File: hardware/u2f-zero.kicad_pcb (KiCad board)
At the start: 2 copper layers, 40.5 x 14.5 mm, 16 parts, among them SW1 SW_PUSH

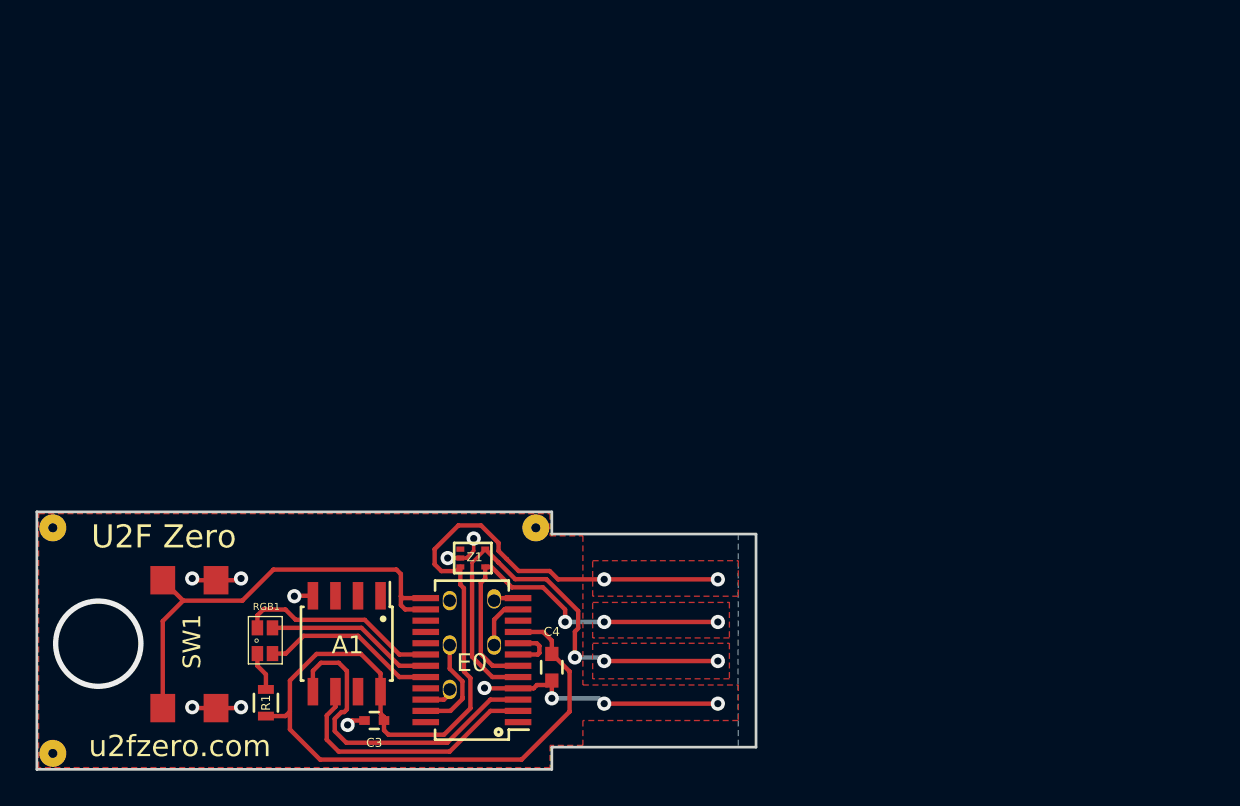
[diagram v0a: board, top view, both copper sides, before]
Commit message: Ensmallen
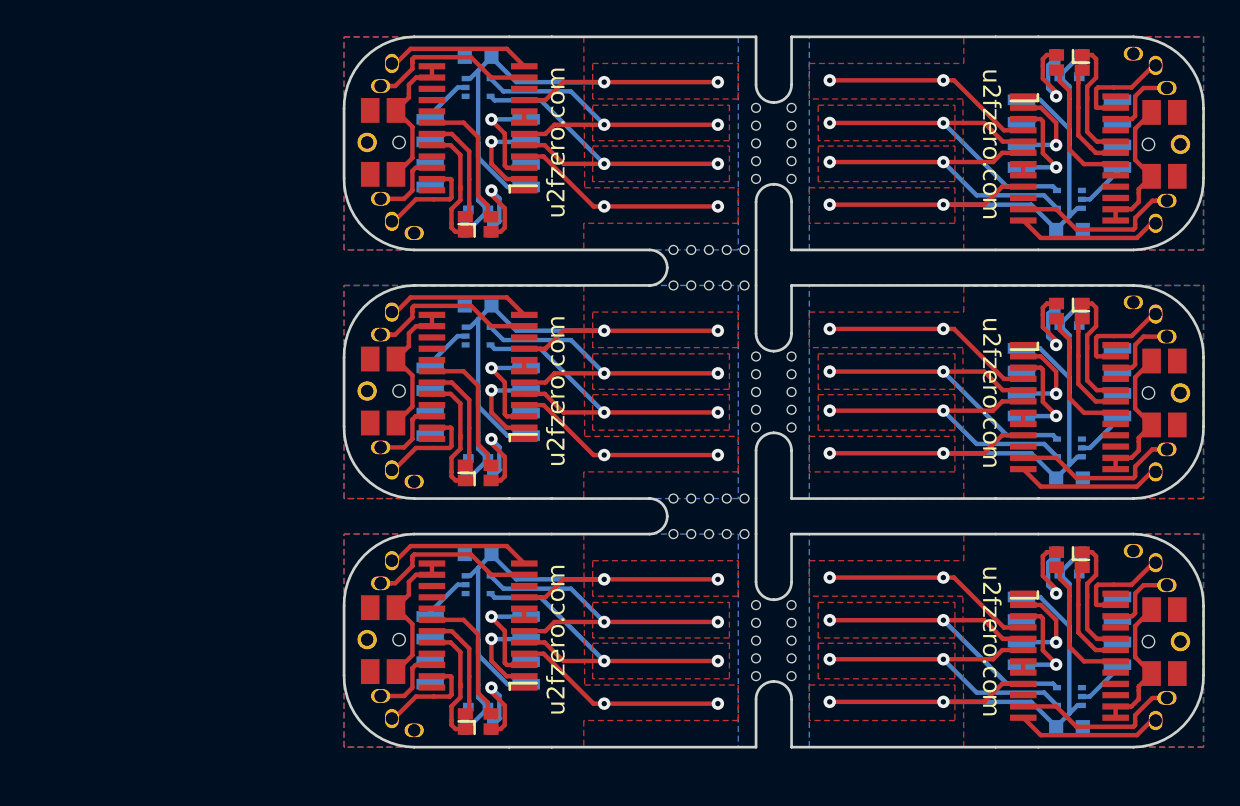
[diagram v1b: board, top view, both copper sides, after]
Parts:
- removed F1, F2, F3: u2f-fiducial, footprints:u2f-fiducial
- removed the SW1 at (43.9, 36.5)
- added A1: ATECC508A, Housings_SOIC:SOIC-8_3.9x4.9mm_Pitch1.27mm, B.Cu at (93.4, 7.70)
- added A1: ATECC508A, Housings_SOIC:SOIC-8_3.9x4.9mm_Pitch1.27mm, B.Cu at (60.1, 8.80)
- added A1: ATECC508A, Housings_SOIC:SOIC-8_3.9x4.9mm_Pitch1.27mm, B.Cu at (60.1, 22.8)
- added A1: ATECC508A, Housings_SOIC:SOIC-8_3.9x4.9mm_Pitch1.27mm, B.Cu at (93.4, 21.7)
- added A1: ATECC508A, Housings_SOIC:SOIC-8_3.9x4.9mm_Pitch1.27mm, B.Cu at (93.4, 35.7)
- added C2CK1: debug-pin, footprints:debug, F.Cu at (98.9, 11.5)
- added C2CK1: debug-pin, footprints:debug, F.Cu at (54.6, 5.02)
- added C2CK1: debug-pin, footprints:debug, F.Cu at (54.6, 19.0)
- added C2CK1: debug-pin, footprints:debug, F.Cu at (98.9, 25.5)
- added C2CK1: debug-pin, footprints:debug, F.Cu at (98.9, 39.5)
- added C2D1: debug-pin, footprints:debug, F.Cu at (98.3, 12.8)
- added C2D1: debug-pin, footprints:debug, F.Cu at (55.2, 3.75)
- added C2D1: debug-pin, footprints:debug, F.Cu at (55.2, 17.8)
- added C2D1: debug-pin, footprints:debug, F.Cu at (98.3, 26.8)
- added C2D1: debug-pin, footprints:debug, F.Cu at (98.3, 40.8)
- added C3: 0.1uF, Capacitors_SMD:C_0402, B.Cu at (93.4, 4.50)
- added C3: 0.1uF, Capacitors_SMD:C_0402, B.Cu at (60.1, 12.0)
- added C3: 0.1uF, Capacitors_SMD:C_0402, B.Cu at (60.1, 26.0)
- added C3: 0.1uF, Capacitors_SMD:C_0402, B.Cu at (93.4, 18.5)
- added C3: 0.1uF, Capacitors_SMD:C_0402, B.Cu at (93.4, 32.5)
- added C4: 4.7uF, Capacitors_SMD:C_0603, B.Cu at (93.4, 13.1)
- added C4: 4.7uF, Capacitors_SMD:C_0603, B.Cu at (60.1, 3.40)
- added C4: 4.7uF, Capacitors_SMD:C_0603, B.Cu at (60.1, 17.4)
- added C4: 4.7uF, Capacitors_SMD:C_0603, B.Cu at (93.4, 27.1)
- added C4: 4.7uF, Capacitors_SMD:C_0603, B.Cu at (93.4, 41.1)
- added E0: EFM8UB1_24pin, footprints:QSOP-24_3.9x8.7mm_Pitch0.635mm_fat, F.Cu at (93.4, 9.10)
- added E0: EFM8UB1_24pin, footprints:QSOP-24_3.9x8.7mm_Pitch0.635mm_fat, F.Cu at (60.1, 7.40)
- added E0: EFM8UB1_24pin, footprints:QSOP-24_3.9x8.7mm_Pitch0.635mm_fat, F.Cu at (60.1, 21.4)
- added E0: EFM8UB1_24pin, footprints:QSOP-24_3.9x8.7mm_Pitch0.635mm_fat, F.Cu at (93.4, 23.1)
- added E0: EFM8UB1_24pin, footprints:QSOP-24_3.9x8.7mm_Pitch0.635mm_fat, F.Cu at (93.4, 37.1)
- added GND1: debug-pin, footprints:debug, F.Cu at (97.0, 3.20)
- added GND1: debug-pin, footprints:debug, F.Cu at (56.5, 13.3)
- added GND1: debug-pin, footprints:debug, F.Cu at (56.5, 27.3)
- added GND1: debug-pin, footprints:debug, F.Cu at (97.0, 17.2)
- added GND1: debug-pin, footprints:debug, F.Cu at (97.0, 31.2)
- added R1: 100, Resistors_SMD:R_0603, B.Cu at (93.4, 3.40)
- added R1: 100, Resistors_SMD:R_0603, B.Cu at (60.1, 13.1)
- added R1: 100, Resistors_SMD:R_0603, B.Cu at (60.1, 27.1)
- added R1: 100, Resistors_SMD:R_0603, B.Cu at (93.4, 17.4)
- added R1: 100, Resistors_SMD:R_0603, B.Cu at (93.4, 31.4)
- added REF**: mousebites, footprints:mousebites, F.Cu at (73.1, 30.2)
- added REF**: mousebites, footprints:mousebites, F.Cu at (75.8, 36.2)
- added REF**: mousebites, footprints:mousebites, F.Cu at (73.1, 28.2)
- added REF**: mousebites, footprints:mousebites, F.Cu at (73.1, 16.2)
- added REF**: mousebites, footprints:mousebites, F.Cu at (73.1, 14.2)
- added REF**: mousebites, footprints:mousebites, F.Cu at (77.8, 8.25)
- added REF**: mousebites, footprints:mousebites, F.Cu at (75.8, 8.25)
- added REF**: mousebites, footprints:mousebites, F.Cu at (75.8, 22.2)
- added REF**: mousebites, footprints:mousebites, F.Cu at (77.8, 22.2)
- added REF**: mousebites, footprints:mousebites, F.Cu at (77.8, 36.2)
- added RGB1: CA_RGB, footprints:LED-0606, F.Cu at (93.4, 3.70)
- added RGB1: CA_RGB, footprints:LED-0606, F.Cu at (60.1, 12.8)
- added RGB1: CA_RGB, footprints:LED-0606, F.Cu at (60.1, 26.8)
- added RGB1: CA_RGB, footprints:LED-0606, F.Cu at (93.4, 17.7)
- added RGB1: CA_RGB, footprints:LED-0606, F.Cu at (93.4, 31.7)
- added RX1: debug-pin, footprints:debug, F.Cu at (98.9, 5.13)
- added RX1: debug-pin, footprints:debug, F.Cu at (54.6, 11.4)
- added RX1: debug-pin, footprints:debug, F.Cu at (54.6, 25.4)
- added RX1: debug-pin, footprints:debug, F.Cu at (98.9, 19.1)
- added RX1: debug-pin, footprints:debug, F.Cu at (98.9, 33.1)
- added SW1: SW_PUSH, Buttons_Switches_SMD:SW_SPST_EVQP7C, F.Cu at (98.8, 8.30)
- added SW1: SW_PUSH, Buttons_Switches_SMD:SW_SPST_EVQP7C, F.Cu at (54.8, 8.20)
- added SW1: SW_PUSH, Buttons_Switches_SMD:SW_SPST_EVQP7C, F.Cu at (54.8, 22.2)
- added SW1: SW_PUSH, Buttons_Switches_SMD:SW_SPST_EVQP7C, F.Cu at (98.8, 22.3)
- added SW1: SW_PUSH, Buttons_Switches_SMD:SW_SPST_EVQP7C, F.Cu at (98.8, 36.3)
- added SW1: SW_PUSH, Buttons_Switches_SMD:SW_SPST_EVQP7C, F.Cu at (54.8, 36.2)
- added TX1: debug-pin, footprints:debug, F.Cu at (98.3, 3.86)
- added TX1: debug-pin, footprints:debug, F.Cu at (55.2, 12.6)
- added TX1: debug-pin, footprints:debug, F.Cu at (55.2, 26.6)
- added TX1: debug-pin, footprints:debug, F.Cu at (98.3, 17.9)
- added TX1: debug-pin, footprints:debug, F.Cu at (98.3, 31.9)
- added Z1: DF5A5.6JE, TO_SOT_Packages_SMD:SOT-553, B.Cu at (93.4, 11.4)
- added Z1: DF5A5.6JE, TO_SOT_Packages_SMD:SOT-553, B.Cu at (60.1, 5.10)
- added Z1: DF5A5.6JE, TO_SOT_Packages_SMD:SOT-553, B.Cu at (60.1, 19.1)
- added Z1: DF5A5.6JE, TO_SOT_Packages_SMD:SOT-553, B.Cu at (93.4, 25.4)
- added Z1: DF5A5.6JE, TO_SOT_Packages_SMD:SOT-553, B.Cu at (93.4, 39.4)
- A1, C3, C4, R1, Z1: moved to B.Cu
- moved RGB1 12.8 mm to (60.1, 40.8), turned to 90 degrees
- moved R1 12.0 mm to (60.1, 41.1), turned to 0 degrees
- moved C4 7.59 mm to (60.1, 31.4), turned to 0 degrees
- moved GND1 7.57 mm to (56.5, 41.3), turned to 270 degrees
- moved A1 7.41 mm to (60.1, 36.8), turned to 0 degrees
- moved C2CK1 7.28 mm to (54.6, 33.0), turned to 90 degrees
- moved C2D1 6.18 mm to (55.2, 31.8), turned to 180 degrees
- moved C3 5.90 mm to (60.1, 40.0)
- moved TX1 5.27 mm to (55.2, 40.6)
- moved RX1 3.91 mm to (54.6, 39.4), turned to 90 degrees
- moved E0 1.98 mm to (60.1, 35.4)
- moved Z1 1.53 mm to (60.1, 33.1)
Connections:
- RGB1 pad 1: Net-(E0-Pad18) -> Net-(E0-Pad20)
- RGB1 pad 3: Net-(E0-Pad20) -> Net-(E0-Pad18)
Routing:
- net /+5V: track 72.3 -> 206.8 mm, vias 2 -> 12
- net /HD+: track 27.0 -> 117.0 mm, vias 3 -> 12
- net /HD-: track 22.2 -> 111.5 mm, vias 3 -> 12
- net GND: track 24.5 -> 92.7 mm
- net /C2CK: track 3.02 -> 57.3 mm
- net /C2D: track 1.41 -> 50.8 mm
- net Net-(E0-Pad18): track 11.4 -> 46.3 mm
- net Net-(R1-Pad2): track 2.22 -> 36.8 mm, vias 0 -> 6
- net Net-(E0-Pad20): track 10.0 -> 42.1 mm
- net /TX: track 5.67 -> 35.5 mm
- net Net-(E0-Pad19): track 9.52 -> 38.3 mm
- net Net-(E0-Pad13): track 25.9 -> 49.3 mm
- net /RX: track 1.73 -> 24.7 mm
- net Net-(A1-Pad6): track 14.9 -> 36.2 mm, vias 0 -> 6
- net Net-(A1-Pad5): track 18.8 -> 36.1 mm, vias 0 -> 6
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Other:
- board size 40.5 x 14.5 mm -> 48.4 x 40 mm
- net class Default: via_dia 0.8 -> 0.7; via_drill 0.4 -> 0.3
- rule pad_to_mask_clearance: 0.1 -> 0
- board text removed: "+5v"
- board text removed: "C2CK"
- board text removed: "C2D"
- board text removed: "D+"
- board text removed: "D-"
- board text removed: "GND"
- board text removed: "RX"
- board text removed: "TX"
- board text removed: "U2F Zero"
